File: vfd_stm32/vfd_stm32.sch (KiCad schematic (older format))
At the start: 7 parts, among them SW1 SW_DIP_x04, U2 DRV8848

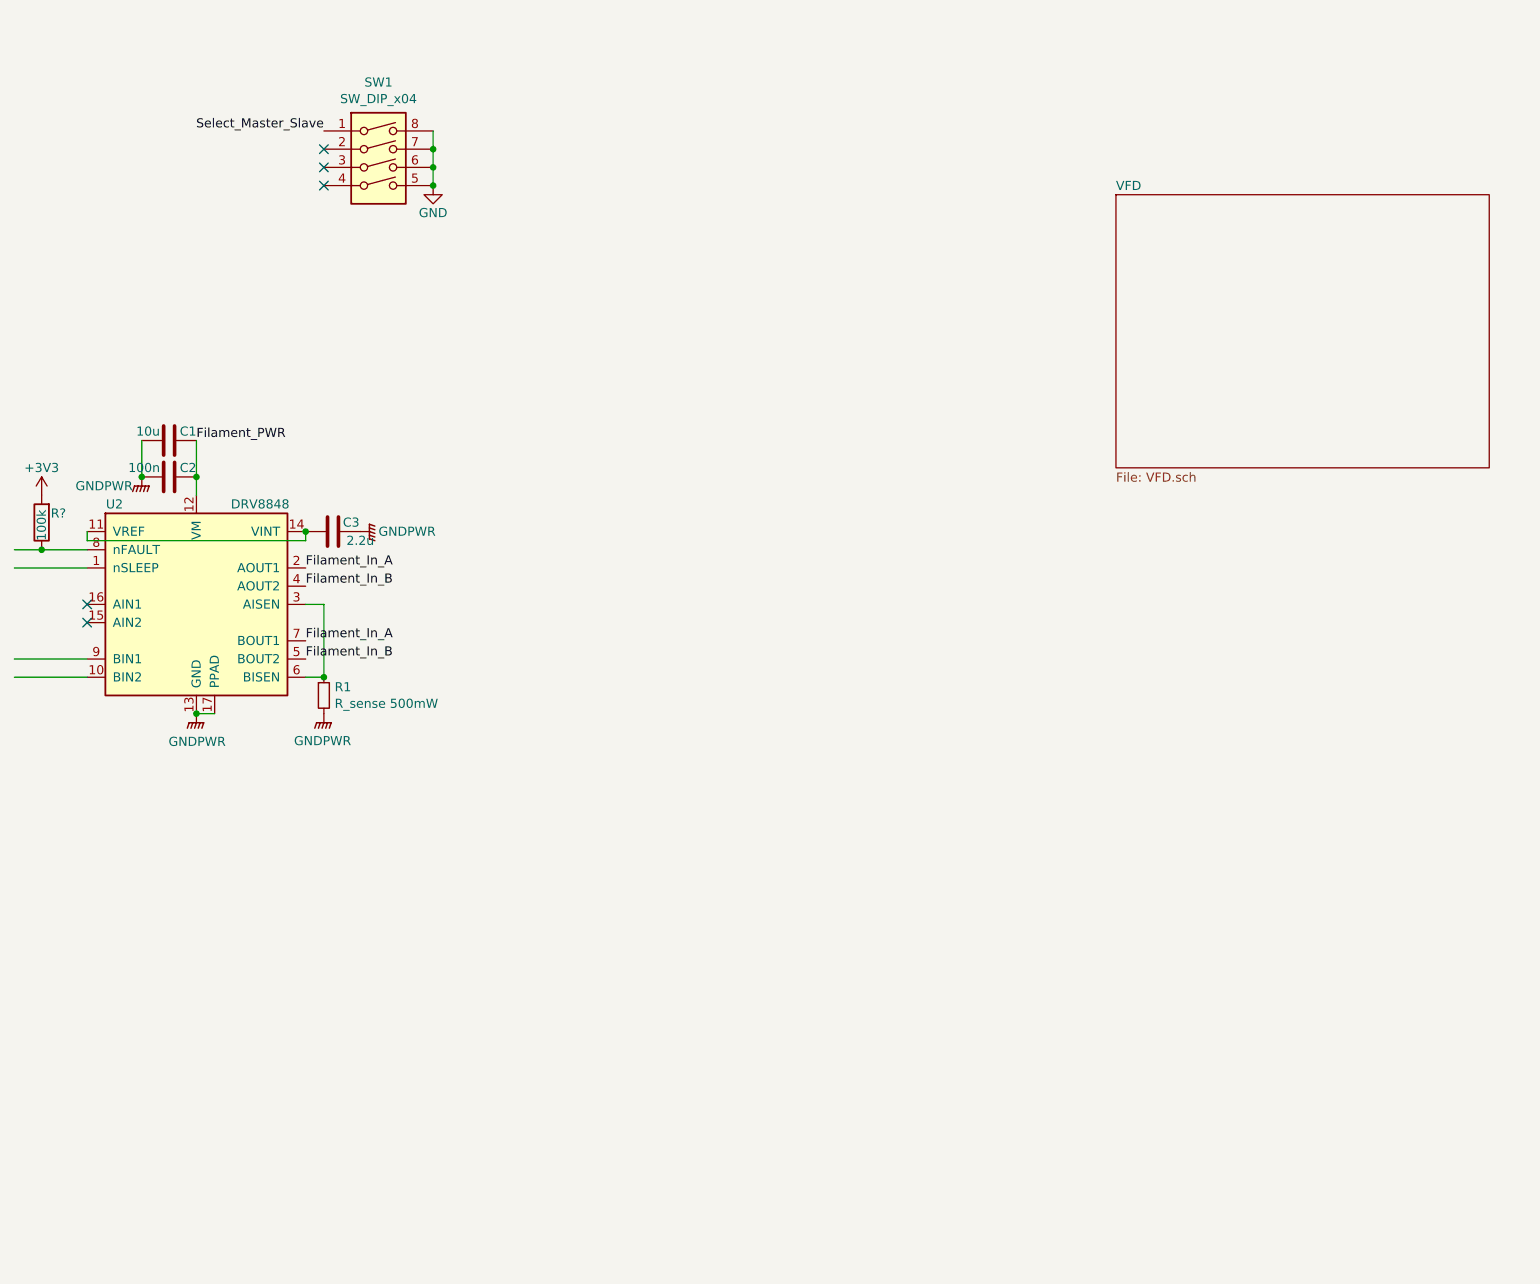
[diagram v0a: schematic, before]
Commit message: cleanup electronics
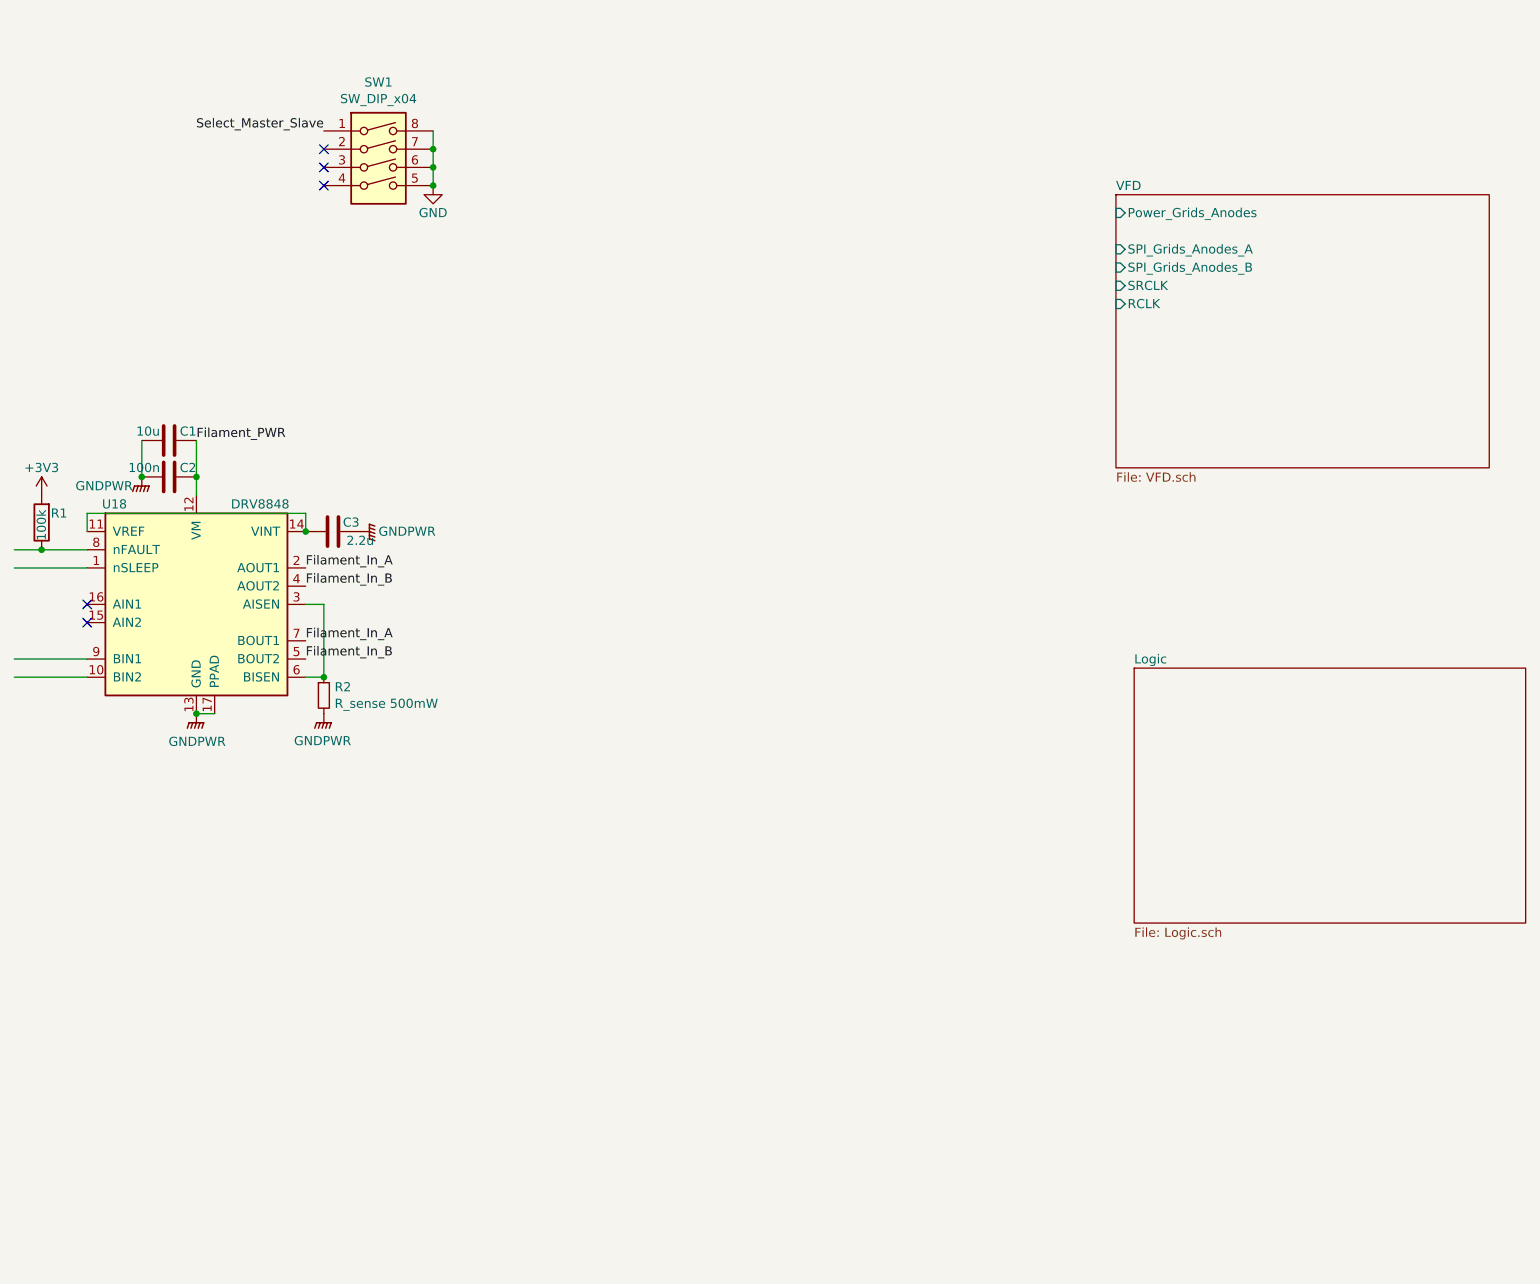
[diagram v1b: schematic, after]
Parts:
- C1: footprint (none) -> Capacitor_SMD:C_1206_3216Metric_Pad1.42x1.75mm_HandSolder
- C2, C3: footprint (none) -> Capacitor_SMD:C_0805_2012Metric_Pad1.15x1.40mm_HandSolder
- R1: renamed from R?; footprint (none) -> Resistor_SMD:R_0805_2012Metric_Pad1.15x1.40mm_HandSolder
- R2: renamed from R1; footprint (none) -> Resistor_SMD:R_1206_3216Metric_Pad1.42x1.75mm_HandSolder
- renumbered U2 to U18
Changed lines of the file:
@@
 EESchema Schematic File Version 4
+LIBS:vfd_stm32-cache
 EELAYER 26 0
 EELAYER END
 $Descr A4 11693 8268
 encoding utf-8
-Sheet 1 2
+Sheet 1 3
 Title ""
 Date ""
@@
 	3700 1050 3700 1150
 $Comp
-L power:GND #PWR03
+L power:GND #PWR06
 U 1 1 5BF6BE22
 P 3700 1150
-F 0 "#PWR03" H 3700 900 50  0001 C CNN
+F 0 "#PWR06" H 3700 900 50  0001 C CNN
 F 1 "GND" H 3700 1000 50  0000 C CNN
 F 2 "" H 3700 1150 50  0001 C CNN
@@
 Connection ~ 3700 1150
 $Comp
-L Driver_Motor:DRV8848 U2
-U 1 1 5BF82047
-P 2400 3450
-F 0 "U2" H 1950 4000 50  0000 C CNN
-F 1 "DRV8848" H 2750 4000 50  0000 C CNN
-F 2 "Package_SO:TSSOP-16-1EP_4.4x5mm_P0.65mm" H 2400 2750 50  0001 C CNN
-F 3 "http://www.ti.com/lit/ds/symlink/drv8848.pdf" H 1250 4800 50  0001 C CNN
-	1    2400 3450
-	1    0    0    -1
-$EndComp
-$Comp
-L power:GNDPWR #PWR02
+L power:GNDPWR #PWR03
 U 1 1 5BF82479
 P 2400 4050
-F 0 "#PWR02" H 2400 3850 50  0001 C CNN
+F 0 "#PWR03" H 2400 3850 50  0001 C CNN
 F 1 "GNDPWR" H 2404 3896 50  0000 C CNN
 F 2 "" H 2400 4000 50  0001 C CNN
@@
 	3000 3850 3100 3850
 $Comp
-L Device:R_Small R1
+L Device:R_Small R2
 U 1 1 5BF8361D
 P 3100 3950
-F 0 "R1" H 3159 3996 50  0000 L CNN
+F 0 "R2" H 3159 3996 50  0000 L CNN
 F 1 "R_sense 500mW" H 3159 3905 50  0000 L CNN
-F 2 "" H 3100 3950 50  0001 C CNN
+F 2 "Resistor_SMD:R_1206_3216Metric_Pad1.42x1.75mm_HandSolder" H 3100 3950 50  0001 C CNN
 F 3 "~" H 3100 3950 50  0001 C CNN
 	1    3100 3950
@@
 F 0 "C3" V 3100 3150 50  0000 C CNN
 F 1 "2.2u" V 3200 3200 50  0000 C CNN
-F 2 "" H 3188 2900 50  0001 C CNN
-F 3 "~" H 3150 3050 50  0001 C CNN
+F 2 "Capacitor_SMD:C_0805_2012Metric_Pad1.15x1.40mm_HandSolder" H 3188 2900 50  0001 C CNN
+F 3 "https://fr.rs-online.com/web/p/condensateurs-ceramique-multicouche/1464271/" H 3150 3050 50  0001 C CNN
 	1    3150 3050
 	0    1    1    0
@@
 	0    -1   -1   0
 $EndComp
-Wire Wire Line
-	3000 3050 3000 3100
-Wire Wire Line
-	3000 3100 1800 3100
-Wire Wire Line
-	1800 3100 1800 3050
-Connection ~ 3000 3050
 $Comp
 L Device:C C2
@@
 F 0 "C2" V 2300 2600 50  0000 L CNN
 F 1 "100n" V 2300 2800 50  0000 L CNN
-F 2 "" H 2288 2600 50  0001 C CNN
+F 2 "Capacitor_SMD:C_0805_2012Metric_Pad1.15x1.40mm_HandSolder" H 2288 2600 50  0001 C CNN
 F 3 "~" H 2250 2750 50  0001 C CNN
 	1    2250 2750
@@
 F 0 "C1" V 2300 2400 50  0000 L CNN
 F 1 "10u" V 2300 2600 50  0000 L CNN
-F 2 "" H 2288 2400 50  0001 C CNN
-F 3 "~" H 2250 2550 50  0001 C CNN
+F 2 "Capacitor_SMD:C_1206_3216Metric_Pad1.42x1.75mm_HandSolder" H 2288 2400 50  0001 C CNN
+F 3 "https://fr.rs-online.com/web/p/condensateurs-ceramique-multicouche/6530620/" H 2250 2550 50  0001 C CNN
 	1    2250 2550
 	0    -1   -1   0
@@
 	2100 2550 2100 2750
 $Comp
-L power:GNDPWR #PWR01
+L power:GNDPWR #PWR02
 U 1 1 5BF844EC
 P 2100 2750
-F 0 "#PWR01" H 2100 2550 50  0001 C CNN
+F 0 "#PWR02" H 2100 2550 50  0001 C CNN
 F 1 "GNDPWR" H 2050 2700 50  0000 R CNN
 F 2 "" H 2100 2700 50  0001 C CNN
@@
 Connection ~ 2100 2750
 $Comp
-L Device:R R?
+L Device:R R1
 U 1 1 5BF84EB9
 P 1550 3000
-F 0 "R?" H 1500 2950 50  0000 R CNN
+F 0 "R1" H 1500 2950 50  0000 R CNN
 F 1 "100k" V 1550 3100 50  0000 R CNN
-F 2 "" V 1480 3000 50  0001 C CNN
+F 2 "Resistor_SMD:R_0805_2012Metric_Pad1.15x1.40mm_HandSolder" V 1480 3000 50  0001 C CNN
 F 3 "~" H 1550 3000 50  0001 C CNN
 	1    1550 3000
@@
 	1550 3150 1800 3150
 $Comp
-L power:+3V3 #PWR?
+L power:+3V3 #PWR01
 U 1 1 5BF855D0
 P 1550 2850
-F 0 "#PWR?" H 1550 2700 50  0001 C CNN
+F 0 "#PWR01" H 1550 2700 50  0001 C CNN
 F 1 "+3V3" H 1550 3000 50  0000 C CNN
 F 2 "" H 1550 2850 50  0001 C CNN
@@
 Wire Wire Line
 	2400 4050 2500 4050
-Connection ~ 2400 4050
 $Sheet
 S 7450 1200 2050 1500
@@
 F0 "VFD" 50
 F1 "VFD.sch" 50
+F2 "SPI_Grids_Anodes_A" I L 7450 1500 50
+F3 "RCLK" I L 7450 1800 50
+F4 "SPI_Grids_Anodes_B" I L 7450 1600 50
+F5 "SRCLK" I L 7450 1700 50
+F6 "Power_Grids_Anodes" I L 7450 1300 50
 $EndSheet
+Connection ~ 3000 3050
+Connection ~ 2400 4050
+$Comp
+L Driver_Motor:DRV8848 U18
+U 1 1 5BF82047
+P 2400 3450
+F 0 "U18" H 1950 4000 50  0000 C CNN
+F 1 "DRV8848" H 2750 4000 50  0000 C CNN
+F 2 "Package_SO:TSSOP-16-1EP_4.4x5mm_P0.65mm" H 2400 2750 50  0001 C CNN
+F 3 "http://www.ti.com/lit/ds/symlink/drv8848.pdf" H 1250 4800 50  0001 C CNN
+	1    2400 3450
+	1    0    0    -1
+$EndComp
+$Sheet
+S 7550 3800 2150 1400
+U 5C025ADD
+F0 "Logic" 50
+F1 "Logic.sch" 50
+$EndSheet
+Wire Wire Line
+	1800 3050 1800 2950
+Wire Wire Line
+	1800 2950 3000 2950
+Wire Wire Line
+	3000 2950 3000 3050
 $EndSCHEMATC

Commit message: routage terminé
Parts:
- removed SW1: SW_DIP_x04, symbol Switch:SW_DIP_x04
- added C12: 33n, Capacitor_SMD:C_0805_2012Metric_Pad1.15x1.40mm_HandSolder, symbol Device:C
- added R3, R4: 100, Resistor_SMD:R_0805_2012Metric_Pad1.15x1.40mm_HandSolder, symbol Device:R
- added R5, R6: 47k, Resistor_SMD:R_0805_2012Metric_Pad1.15x1.40mm_HandSolder, symbol Device:R
- added U19: TSZ121ILT, Package_TO_SOT_SMD:SOT-23-5, symbol Amplifier_Operational:NCS325
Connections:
- net labels added: Filament_ADC, VCC, VDD, VSS
- net labels removed: GNDPWR, Select_Master_Slave
- wire segments 18 -> 32
- no-connect marks 5 -> 2
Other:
- moved on the sheet: C1, C2, C3, R1, R2, U18

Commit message: remove global labels
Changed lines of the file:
@@
 Wire Wire Line
 	1950 6150 1550 6150
-Wire Wire Line
-	2550 6350 2650 6350
 $Sheet
 S 7450 1200 2050 1500
@@
 F0 "VFD" 50
 F1 "VFD.sch" 50
-F2 "SPI_Grids_Anodes_A" I L 7450 1500 50
-F3 "RCLK" I L 7450 1800 50
-F4 "SPI_Grids_Anodes_B" I L 7450 1600 50
-F5 "SRCLK" I L 7450 1700 50
-F6 "Power_Grids_Anodes" I L 7450 1300 50
+F2 "SPI_Grids_Anodes" I L 7450 1500 50
+F3 "RCLK" I L 7450 1700 50
+F4 "SRCLK" I L 7450 1600 50
+F5 "Power_Grids_Anodes" I L 7450 1300 50
+F6 "Filament_In_B" I L 7450 2100 50
+F7 "Filament_In_A" I L 7450 2000 50
 $EndSheet
 Connection ~ 3150 5350
@@
 	1    0    0    -1
 $EndComp
-Connection ~ 2550 6350
 $Comp
 L power:GND #PWR0133
@@
 	1    0    0    -1
 $EndComp
-Text GLabel 3150 5950 2    50   Input ~ 0
-Filament_In_A
-Text GLabel 3150 6050 2    50   Input ~ 0
-Filament_In_B
-Text GLabel 3150 5550 2    50   Input ~ 0
-Filament_In_A
-Text GLabel 3150 5650 2    50   Input ~ 0
-Filament_In_B
 $Comp
 L power:VCC #PWR0137
@@
 Wire Wire Line
 	2850 900  3050 900
+Connection ~ 2550 6350
+Wire Wire Line
+	2550 6350 2650 6350
+Text Label 3150 5550 0    50   ~ 0
+Filament_In_A
+Text Label 3150 5650 0    50   ~ 0
+Filament_In_B
+Text Label 3150 5950 0    50   ~ 0
+Filament_In_A
+Text Label 3150 6050 0    50   ~ 0
+Filament_In_B
+Text Label 7450 2000 2    50   ~ 0
+Filament_In_A
+Text Label 7450 2100 2    50   ~ 0
+Filament_In_B
 $EndSCHEMATC
